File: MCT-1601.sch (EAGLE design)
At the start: 14 parts, among them J1 DUT, J2 Button, J3 D I/O, J5 A In, J6 Pwr, Q1 BC327

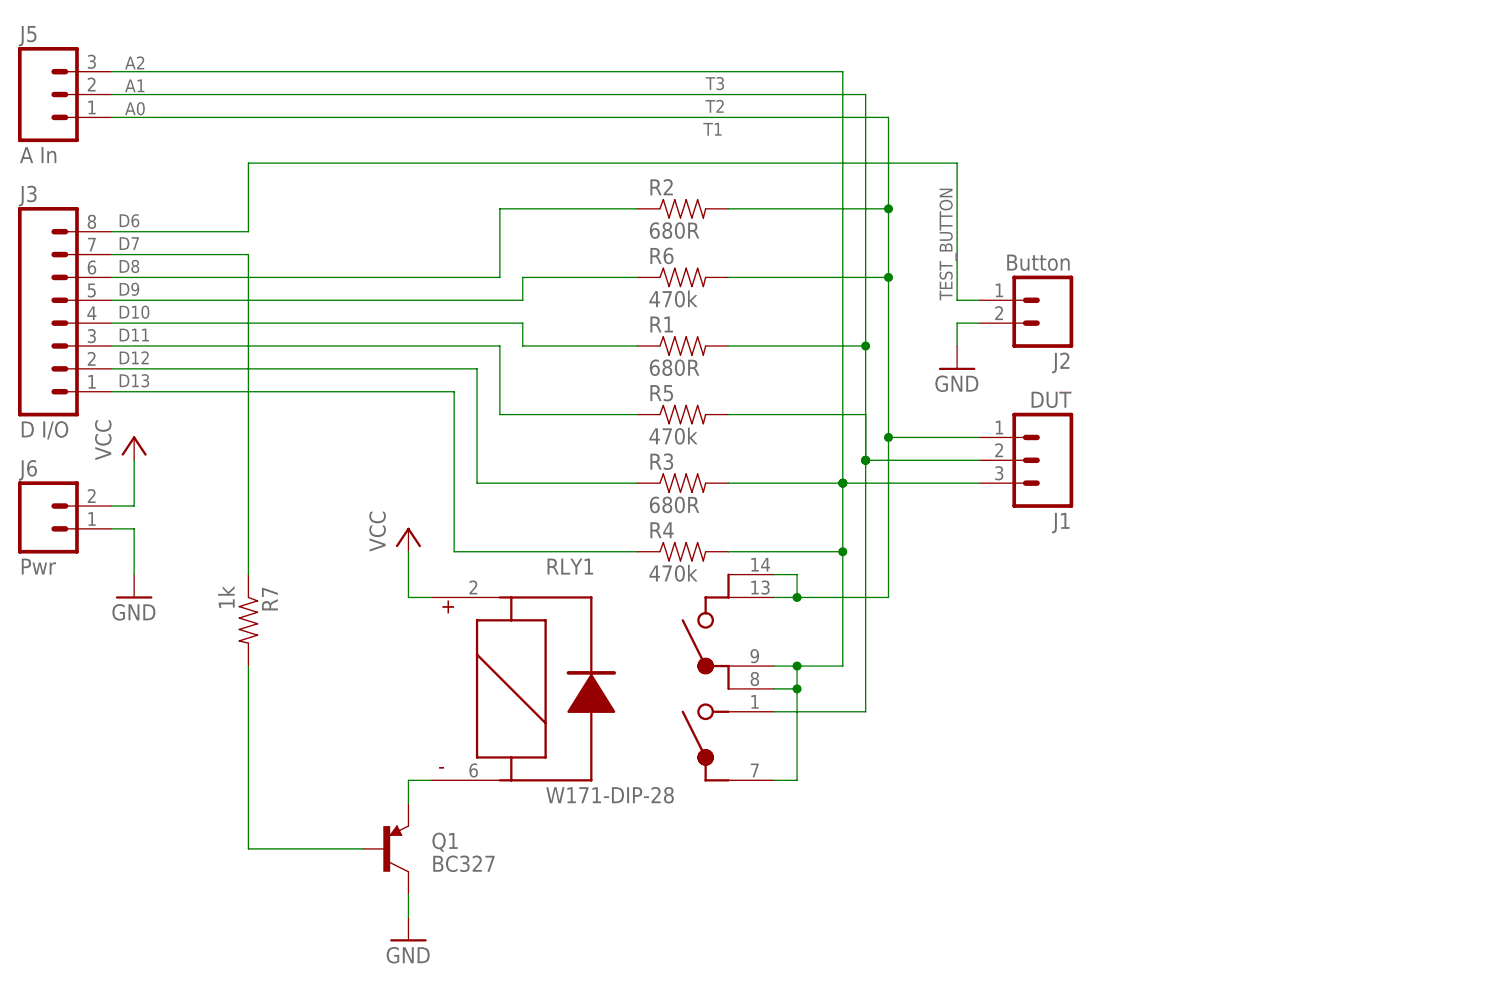
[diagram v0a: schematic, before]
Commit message: Add files via upload
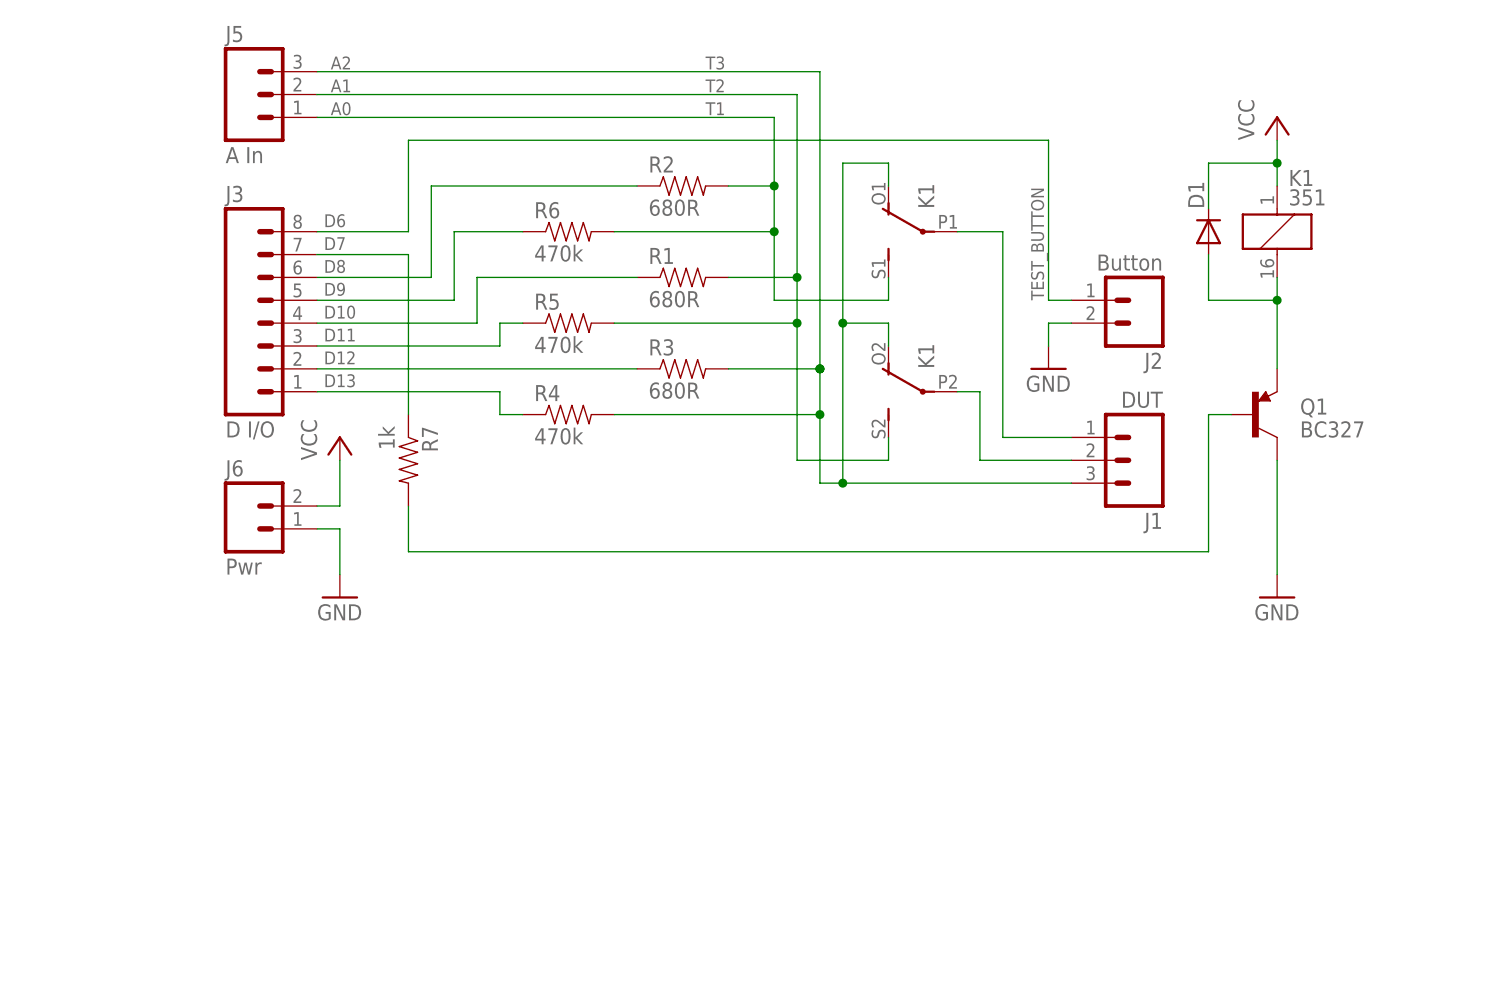
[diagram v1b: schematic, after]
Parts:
- removed RLY1: W171-DIP-28, 00 Nik misc:W171-DIP-28
- added D1: (no value), diode:DIODE-D-2.5
- added K1: 351, relay:351
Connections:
- new net N$1: J1.2, K13.P
- new net N$4: J1.1, K12.P
- net N$3: now also D1.A, K11.2; no longer RLY1.-
- net T1: now also K12.S; no longer J1.1, RLY1.NC2A@1, RLY1.NC2A@2
- net T2: now also K13.S; no longer J1.2, RLY1.NC1A
- net T3: now also K12.O, K13.O; no longer RLY1.NC1B, RLY1.NC2B@1, RLY1.NC2B@2
- net VCC: now also D1.C, K11.1; no longer RLY1.+
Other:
- moved on the sheet: J1, J2, J3, J5, J6, Q1, R1, R2, R3, R4, R5, R6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

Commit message: Add files via upload
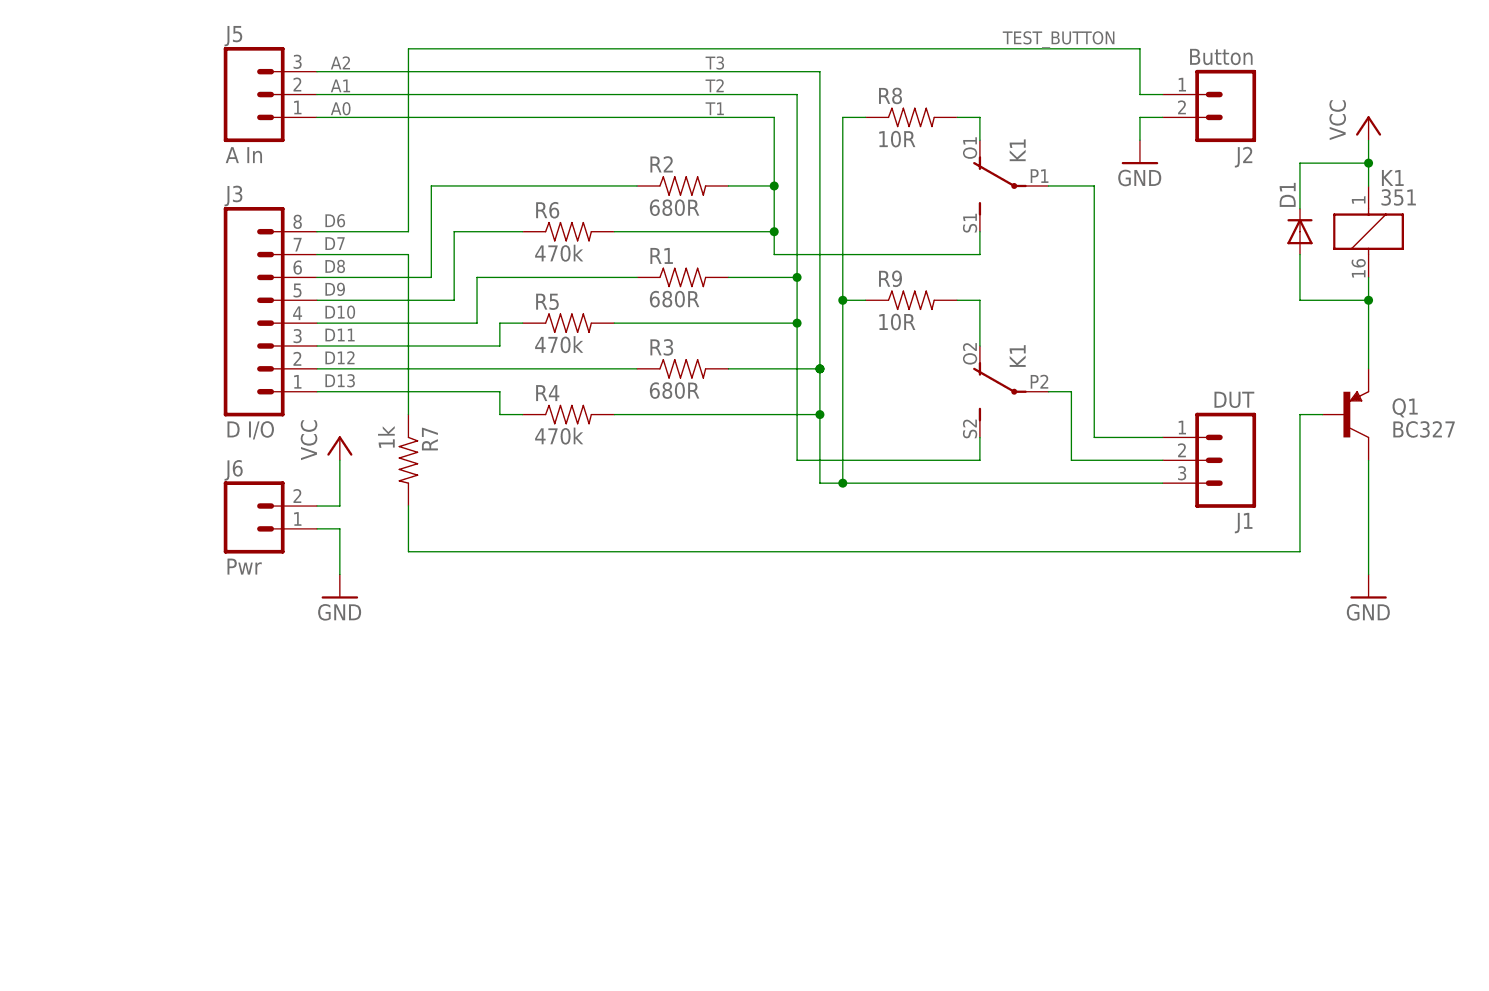
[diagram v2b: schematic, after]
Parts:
- added R8, R9: 10R, SparkFun-Resistors:1KOHM-1/4W-1%(PTH)VERT
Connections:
- new net N$5: K12.O, R8.2
- new net N$6: K13.O, R9.2
- net T3: now also R8.1, R9.1; no longer K12.O, K13.O
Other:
- moved on the sheet: D1, J1, J2, K1, Q1
